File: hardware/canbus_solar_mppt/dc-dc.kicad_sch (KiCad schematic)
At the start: 25 parts

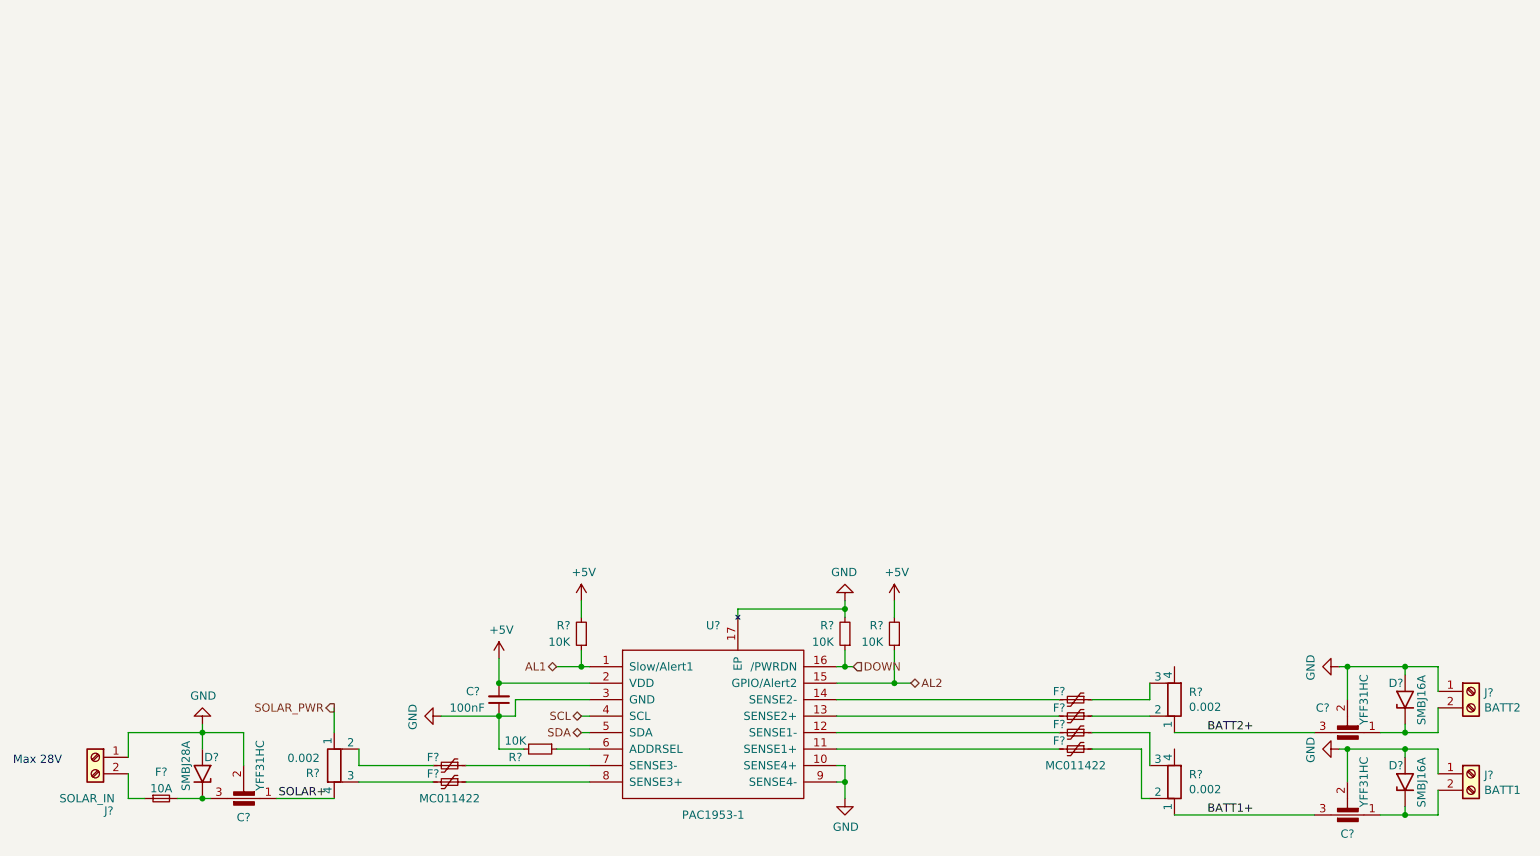
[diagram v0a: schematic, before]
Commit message: WIP: complete DC/DC engine
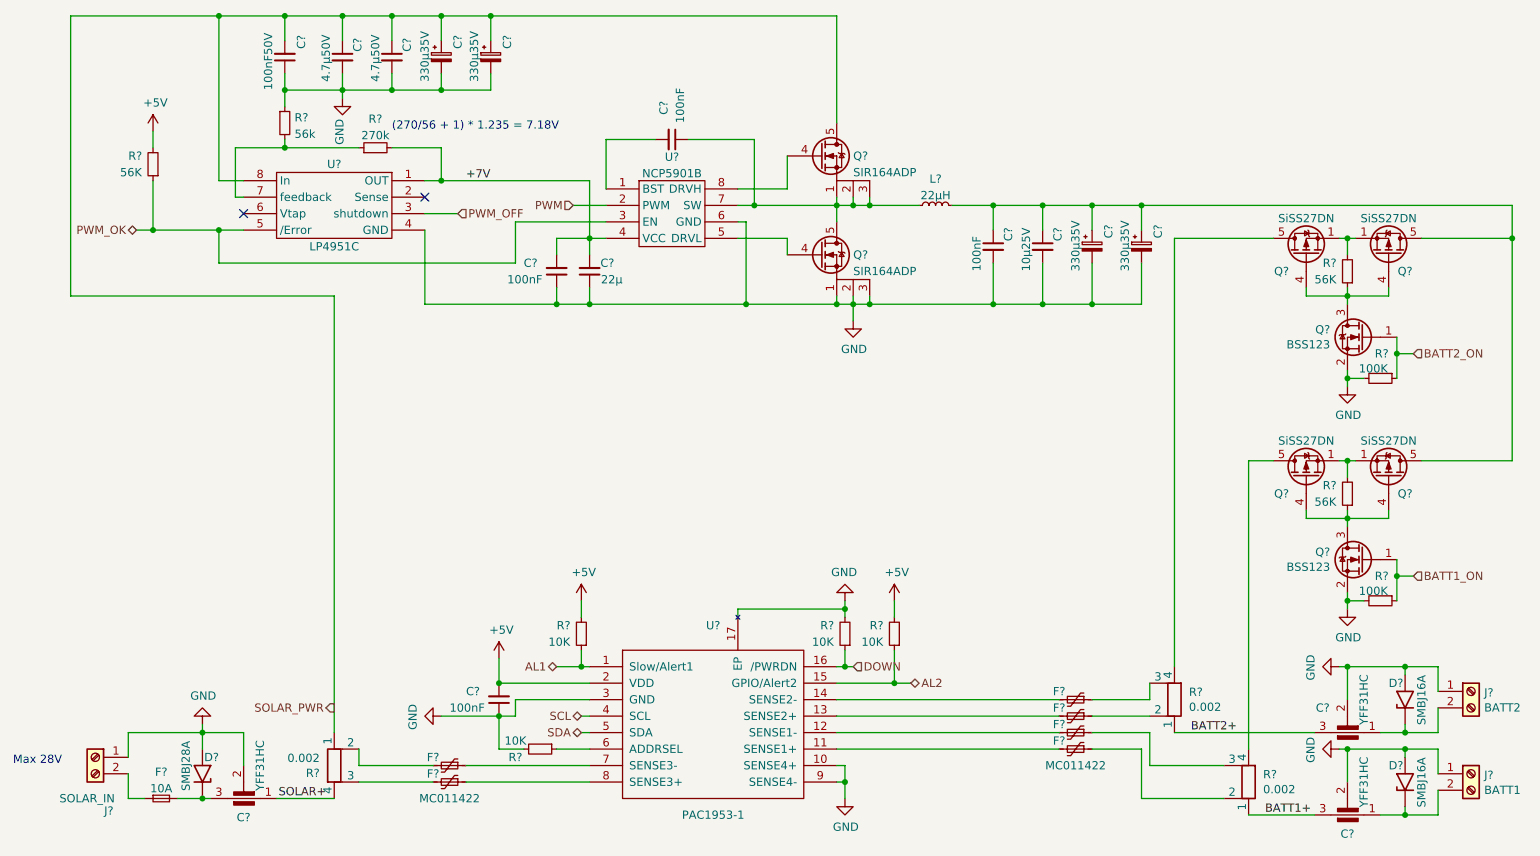
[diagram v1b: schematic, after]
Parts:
- added C?: 10µ25V, Capacitor_SMD:C_1206_3216Metric_Pad1.33x1.80mm_HandSolder, symbol Device:C_Small
- added C? (x4): 330µ35V, Capacitor_SMD:CP_Elec_10x12.6, symbol Device:C_Polarized_Small
- added C? (x2): 100nF, Capacitor_SMD:C_0805_2012Metric_Pad1.18x1.45mm_HandSolder, symbol Device:C_Small
- added C? (x2): 4.7µ50V, Capacitor_SMD:C_1206_3216Metric_Pad1.33x1.80mm_HandSolder, symbol Device:C_Small
- added C?: 100nF, Capacitor_SMD:C_1206_3216Metric_Pad1.33x1.80mm_HandSolder, symbol Device:C_Small
- added C?: 100nF50V, Capacitor_SMD:C_0805_2012Metric_Pad1.18x1.45mm_HandSolder, symbol Device:C_Small
- added C?: 22µ, Capacitor_SMD:C_1206_3216Metric_Pad1.33x1.80mm_HandSolder, symbol Device:C_Small
- added L?: 22µH, Inductor_THT:L_Toroid_Horizontal_D32.5mm_P30.00mm_Bourns_2300, symbol Device:L_Small
- added Q? (x2): SIR164ADP, Package_SO:PowerPAK_SO-8_Single, symbol q_nmos_sssgd:Q_NMOS_SSSGD
- added Q? (x2): BSS123, Package_TO_SOT_SMD:SOT-23, symbol Device:Q_NMOS_GSD
- added Q? (x4): SiSS27DN, Package_SO:Vishay_PowerPAK_1212-8_Single, symbol Transistor_FET:SiSS27DN
- added R? (x3): 56K, Resistor_THT:R_Axial_DIN0207_L6.3mm_D2.5mm_P7.62mm_Horizontal, symbol Device:R_Small
- added R? (x2): 100K, Resistor_THT:R_Axial_DIN0207_L6.3mm_D2.5mm_P7.62mm_Horizontal, symbol Device:R_Small
- added R?: 270k, Resistor_SMD:R_0805_2012Metric_Pad1.20x1.40mm_HandSolder, symbol Device:R_Small
- added R?: 56k, Resistor_SMD:R_0805_2012Metric_Pad1.20x1.40mm_HandSolder, symbol Device:R_Small
- added U?: NCP5901B, Package_SO:SOIC-8_3.9x4.9mm_P1.27mm, symbol onsemi-local:NCP5901B
- added U?: LP4951C, Package_SO:SOIC-8_3.9x4.9mm_P1.27mm, symbol texas-local:LP4951C
- F? (x6): P/N (none) -> MC011422
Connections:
- net +5V: now also R?.2
- net GND: now also C?.1, C?.1, C?.1, C?.2, C?.2, C?.2, C?.2, C?.2, C?.2, C?.2, C?.2, Q?.1 (S), Q?.2 (S), Q?.2 (S), Q?.2 (S), Q?.3 (S), R?.1, R?.2, R?.2, U?.4 (GND), U?.6 (GND)
- net SOLAR_PWR: now also C?.1, C?.1, C?.1, C?.1, C?.2, Q?.5 (D), U?.8 (In)
- net at R?.4: now also Q?.5 (D) (x2)
- new net: C?.1, C?.1, C?.1, C?.1, L?.2, Q?.5 (D), Q?.5 (D)
- new net: C?.2, U?.1 (BST)
- new net: Q?.4 (G), U?.5 (DRVL)
- new net: C?.1, L?.1, Q?.1 (S), Q?.2 (S), Q?.3 (S), Q?.5 (D), U?.7 (SW)
- new net: Q?.4 (G), U?.8 (DRVH)
- new net: Q?.3 (D), Q?.4 (G), Q?.4 (G), R?.1 (x2)
- new net: Q?.1 (S), Q?.1 (S), Q?.2 (S), Q?.2 (S), Q?.3 (S), Q?.3 (S), R?.2 (x2)
- new net: R?.1, R?.2, U?.7 (feedback)
- new net +7V: C?.2, C?.2, R?.2, U?.1 (OUT), U?.4 (VCC)
- new net BATT1_ON: Q?.1 (G), R?.1
- new net BATT2_ON: Q?.1 (G), R?.1
- new net PWM: U?.2 (PWM)
- new net PWM_OFF: U?.3 (shutdown)
- new net PWM_OK: R?.1, U?.3 (EN), U?.5 (/Error)
- no-connect marks 0 -> 2
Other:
- note added: "(270/56 + 1) * 1.235 = 7.18V"
- moved on the sheet: R?
